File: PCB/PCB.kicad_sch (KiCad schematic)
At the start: 54 parts, among them J1 Conn_02x06_Counter_Clockwise, J2 Conn_02x06_Counter_Clockwise, SW1 SW_Push, SW10 SW_Push, SW11 SW_Push, SW12 SW_Push, SW13 SW_Push, SW14 SW_Push, SW15 SW_Push, SW16 SW_Push, SW17 SW_Push, SW2 SW_Push, SW3 SW_Push, SW4 SW_Push, SW5 SW_Push, SW6 SW_Push, SW7 SW_Push, SW8 SW_Push, SW9 SW_Push, U1 MCU_Seeed_XIAO_RP2040

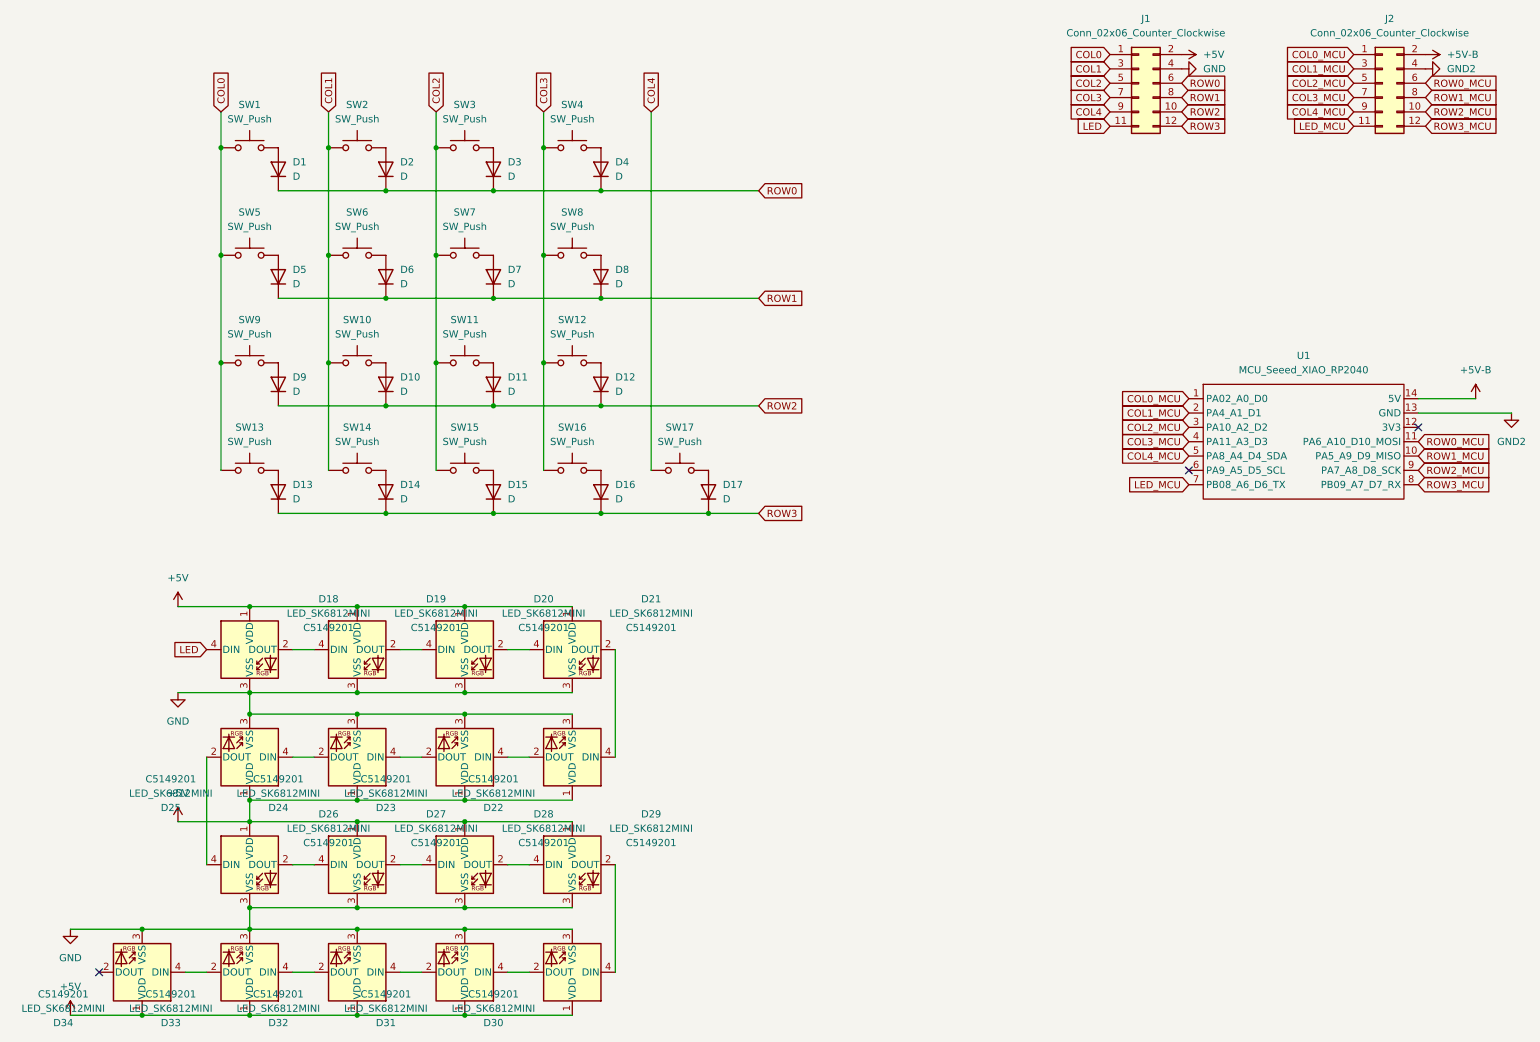
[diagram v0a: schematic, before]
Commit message: added cad files and gerbers
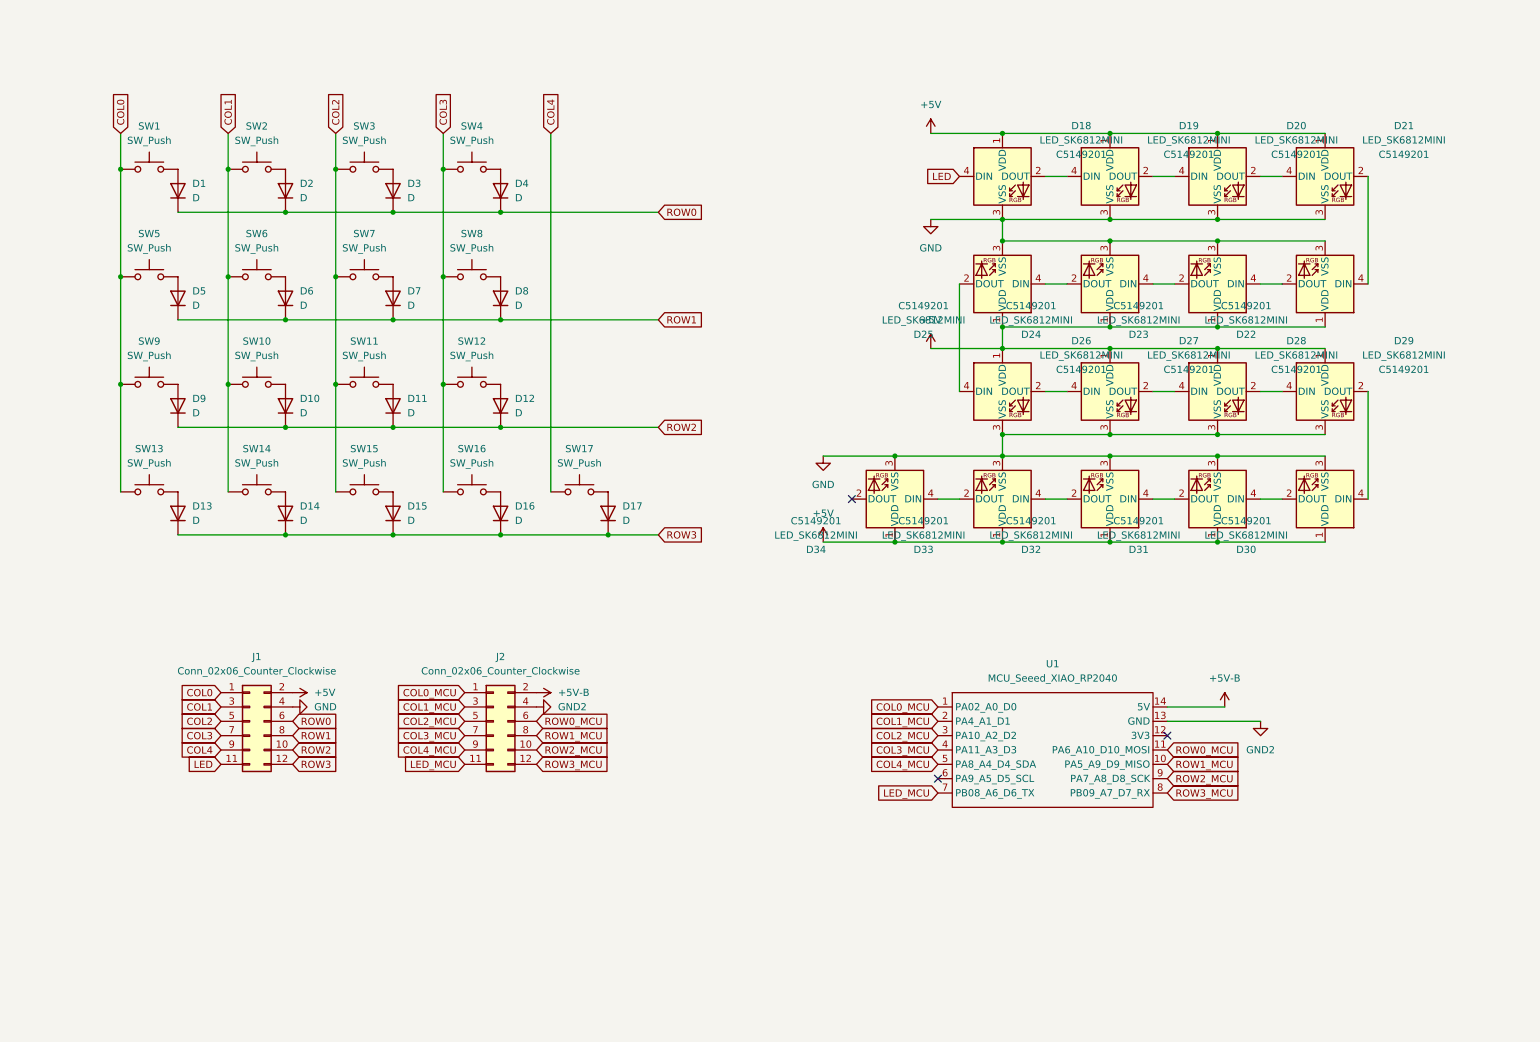
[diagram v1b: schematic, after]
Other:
- moved on the sheet: D1, D10, D11, D12, D13, D14, D15, D16, D17, D18, D19, D2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
